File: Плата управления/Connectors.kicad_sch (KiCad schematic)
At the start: 8 parts, among them J1 Sensor, J12 Power, J2 CAN2, J3 CAN1, J4 A, J5 B, J6 C, J7 RS485

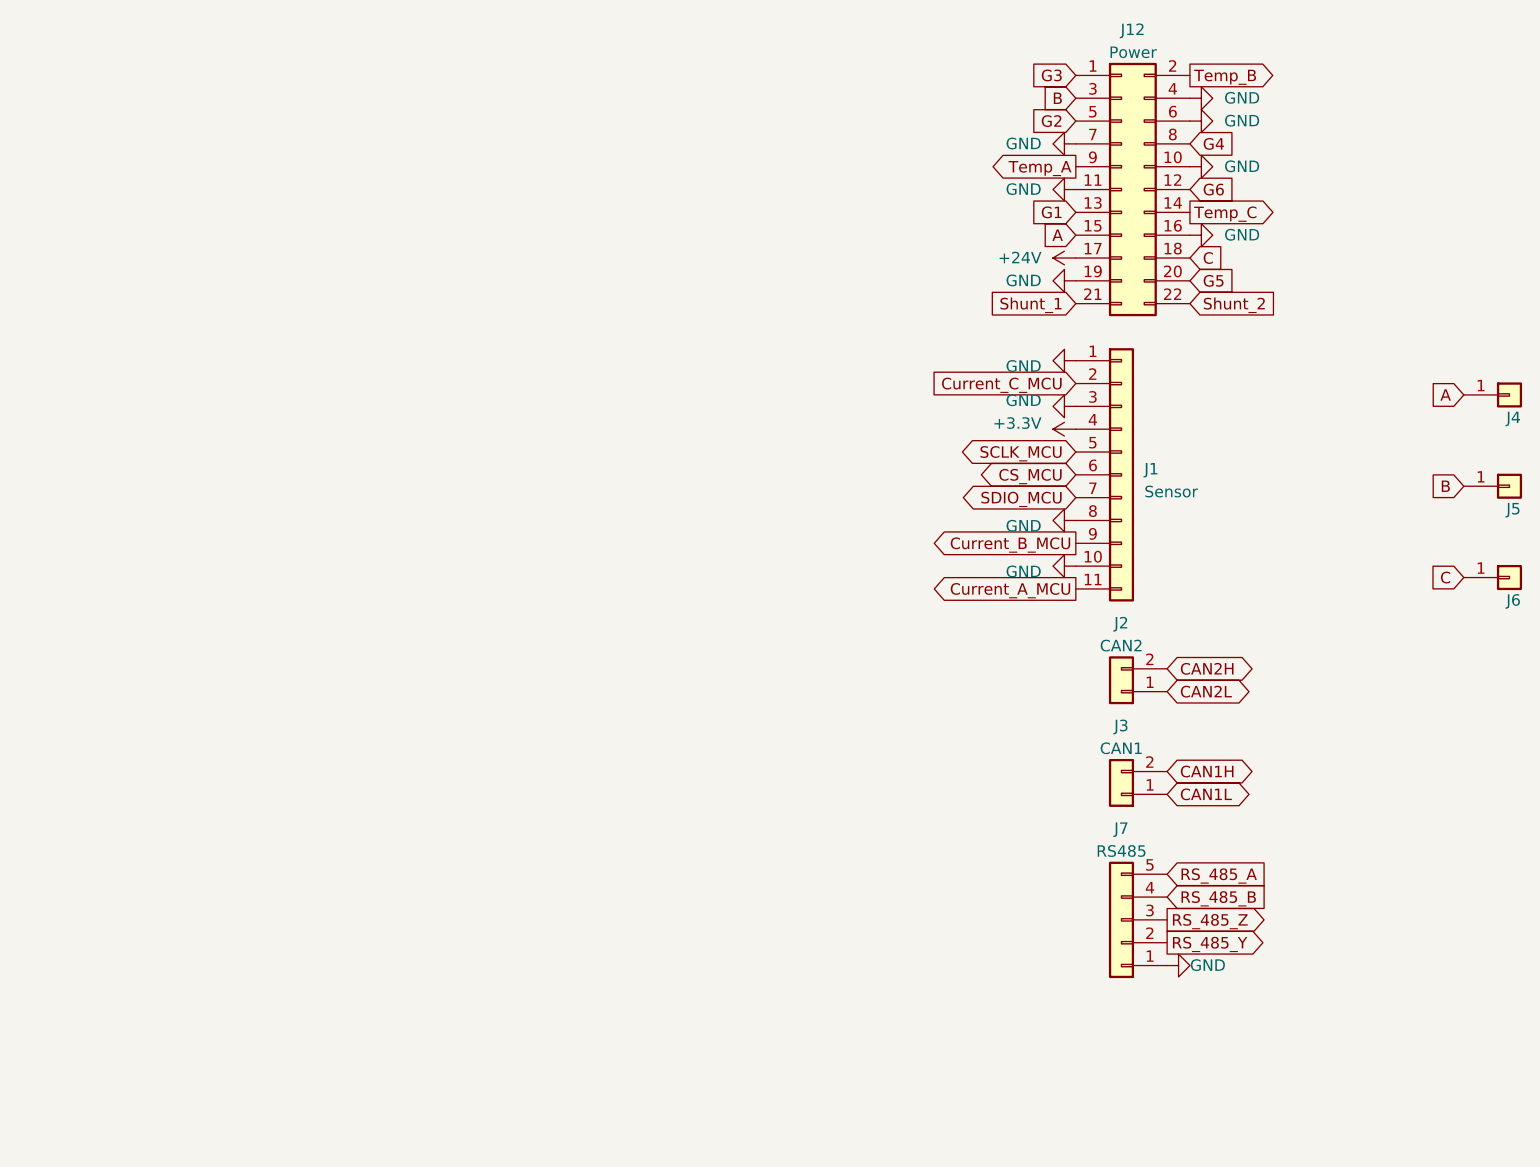
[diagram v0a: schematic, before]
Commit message: Новый контур платы
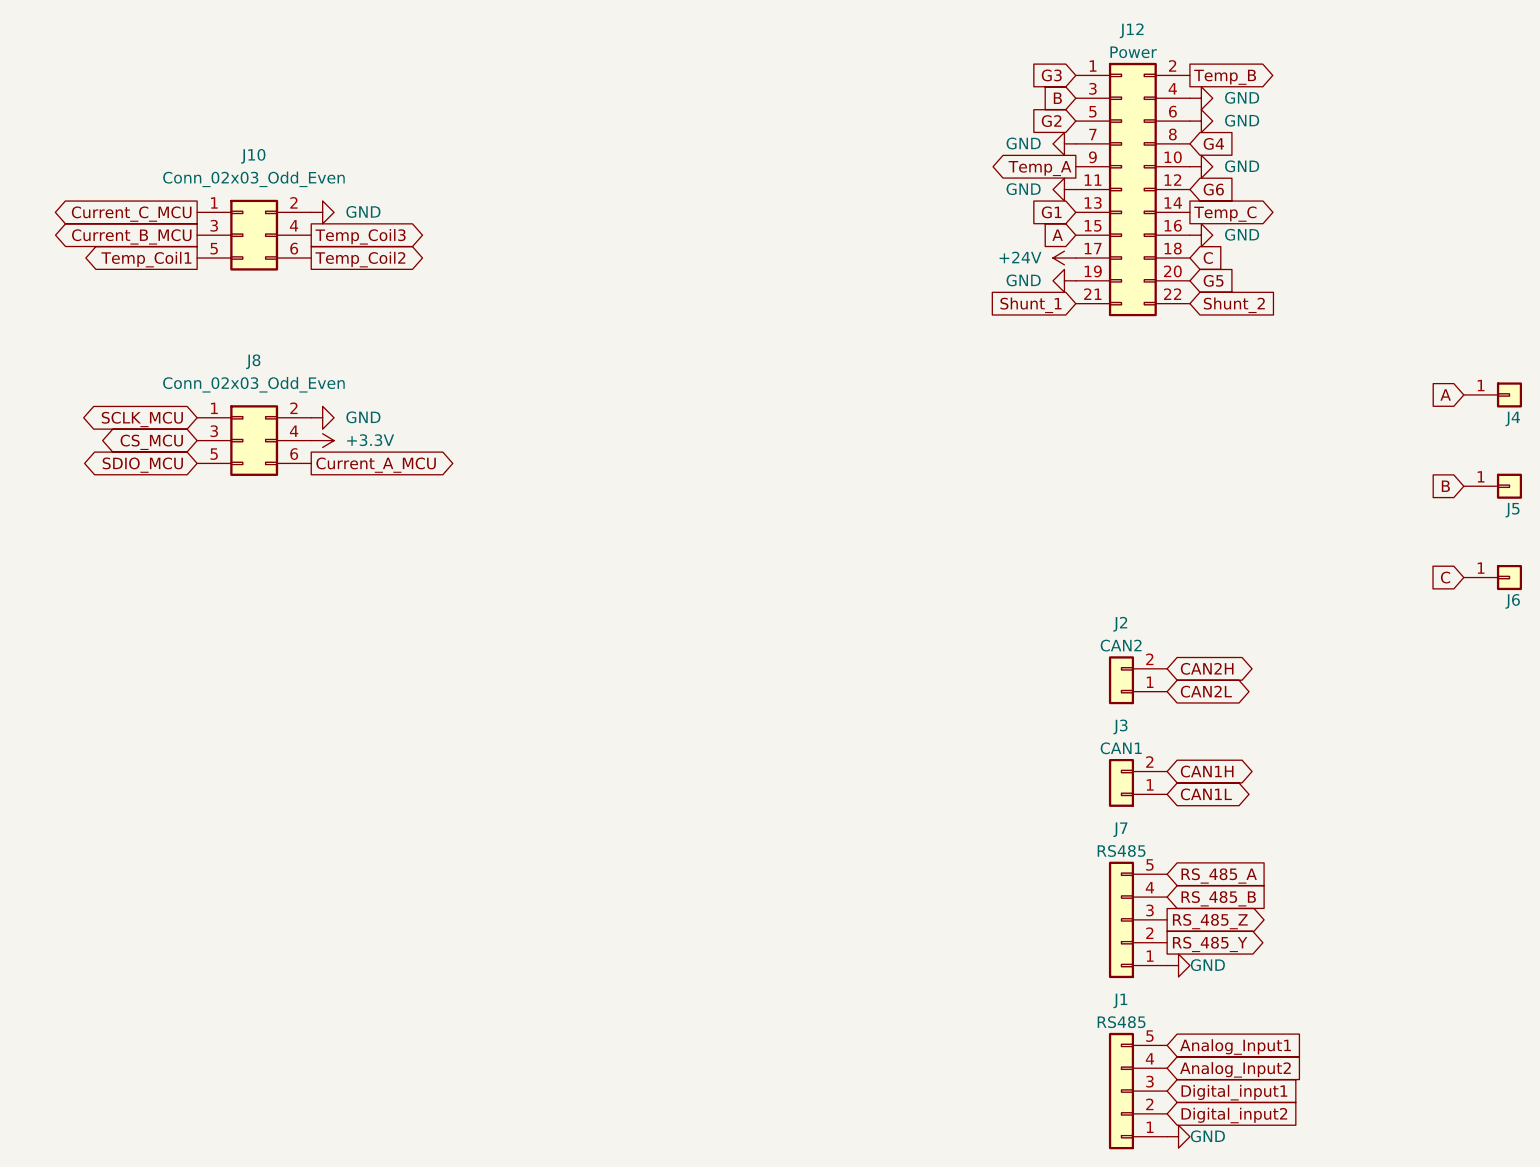
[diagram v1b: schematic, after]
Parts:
- removed J1: Sensor, Connector_PinHeader_2.54mm:PinHeader_1x11_P2.54mm_Vertical, symbol Connector_Generic:Conn_01x11
- added J1: RS485, Connector_Molex:Molex_PicoBlade_53048-0510_1x05_P1.25mm_Horizontal, symbol Connector_Generic:Conn_01x05
- added J10, J8: Conn_02x03_Odd_Even, Connector_PinHeader_2.54mm:PinHeader_2x03_P2.54mm_Vertical_SMD, symbol Connector_Generic:Conn_02x03_Odd_Even
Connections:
- net +3.3V: now also J8.4 (Pin_4)
- net CS_MCU: now also J8.3 (Pin_3)
- net Current_A_MCU: now also J8.6 (Pin_6)
- net Current_B_MCU: now also J10.3 (Pin_3)
- net Current_C_MCU: now also J10.1 (Pin_1)
- net GND: now also J1.1 (Pin_1), J10.2 (Pin_2), J8.2 (Pin_2)
- net SCLK_MCU: now also J8.1 (Pin_1)
- net SDIO_MCU: now also J8.5 (Pin_5)
- new net Analog_Input1: J1.5 (Pin_5)
- new net Analog_Input2: J1.4 (Pin_4)
- new net Digital_input1: J1.3 (Pin_3)
- new net Digital_input2: J1.2 (Pin_2)
- new net Temp_Coil1: J10.5 (Pin_5)
- new net Temp_Coil2: J10.6 (Pin_6)
- new net Temp_Coil3: J10.4 (Pin_4)
